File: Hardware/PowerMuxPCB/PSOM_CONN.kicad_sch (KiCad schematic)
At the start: 31 parts, among them J1 SLIMSTACK, Q2 SQ2315CES-T1_GE3, Q3 SQ2315CES-T1_GE3, Q4 SQ2315CES-T1_GE3, Q5 SQ2315CES-T1_GE3, Q6 SQ2315CES-T1_GE3, Q7 SQ2315CES-T1_GE3

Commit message: silk + roosters
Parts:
- Q2, Q3, Q4, Q5, Q6, Q7: footprint footprints1:PMOSGSD_SOT-23_TO-236_VIS -> PMOSGSD_SOT-23_TO-236_VIS
- TP11: footprint TestPoint:TestPoint_Pad_D2.0mm -> TestPoint:TestPoint_THTPad_D2.0mm_Drill1.0mm
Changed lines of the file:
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@@
 			)
 		)
-		(property "Footprint" "TestPoint:TestPoint_Pad_D2.0mm"
+		(property "Footprint" "TestPoint:TestPoint_THTPad_D2.0mm_Drill1.0mm"
 			(at 144.78 77.47 0)
 			(effects
@@
 			)
 		)
-		(property "Footprint" "footprints1:PMOSGSD_SOT-23_TO-236_VIS"
+		(property "Footprint" "PMOSGSD_SOT-23_TO-236_VIS"
 			(at 208.28 49.53 0)
 			(effects
@@
 			)
 		)
-		(property "Footprint" "footprints1:PMOSGSD_SOT-23_TO-236_VIS"
+		(property "Footprint" "PMOSGSD_SOT-23_TO-236_VIS"
 			(at 208.28 24.13 0)
 			(effects
@@
 			)
 		)
-		(property "Footprint" "footprints1:PMOSGSD_SOT-23_TO-236_VIS"
+		(property "Footprint" "PMOSGSD_SOT-23_TO-236_VIS"
 			(at 184.15 24.13 0)
 			(effects
@@
 			)
 		)
-		(property "Footprint" "footprints1:PMOSGSD_SOT-23_TO-236_VIS"
+		(property "Footprint" "PMOSGSD_SOT-23_TO-236_VIS"
 			(at 184.15 49.53 0)
 			(effects
@@
 			)
 		)
-		(property "Footprint" "footprints1:PMOSGSD_SOT-23_TO-236_VIS"
+		(property "Footprint" "PMOSGSD_SOT-23_TO-236_VIS"
 			(at 208.28 36.83 0)
 			(effects
@@
 			)
 		)
-		(property "Footprint" "footprints1:PMOSGSD_SOT-23_TO-236_VIS"
+		(property "Footprint" "PMOSGSD_SOT-23_TO-236_VIS"
 			(at 184.15 36.83 0)
 			(effects

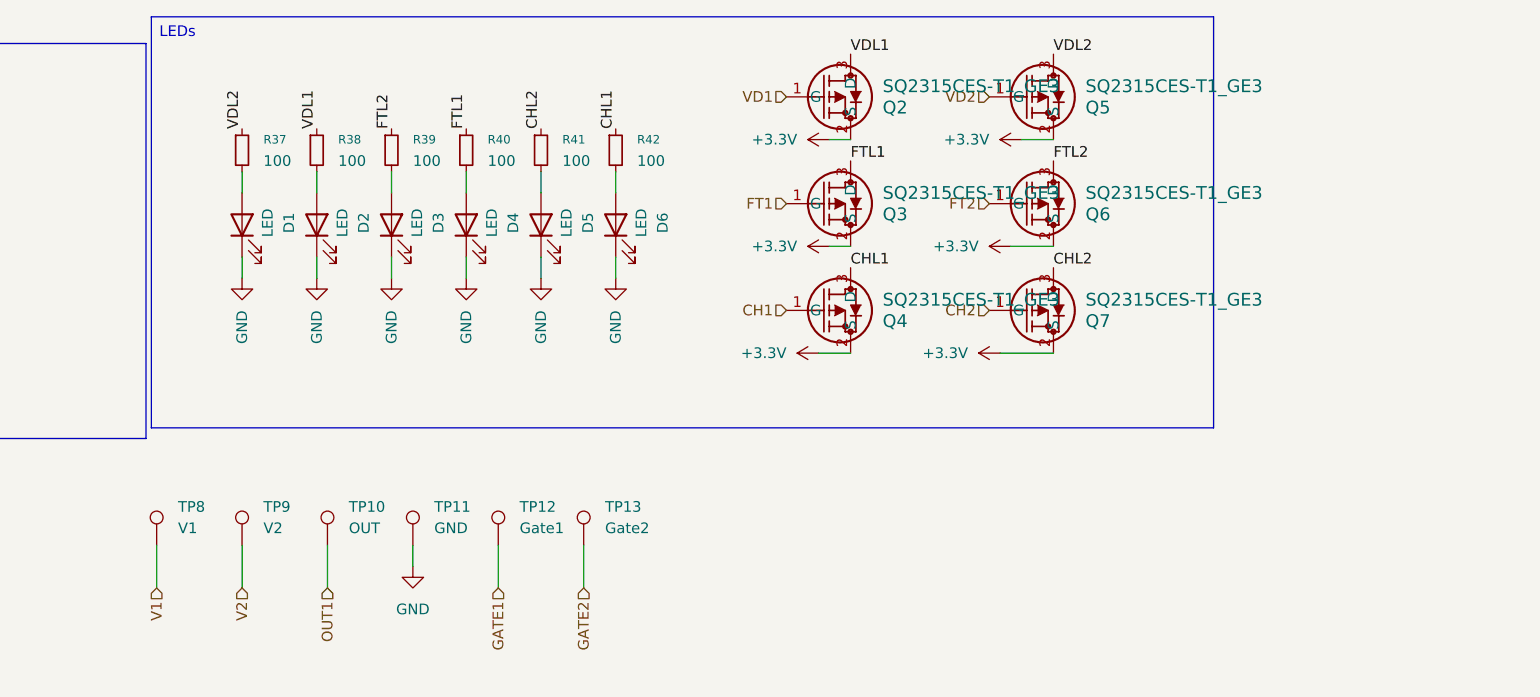
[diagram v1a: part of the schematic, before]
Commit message: cleaned up power mux
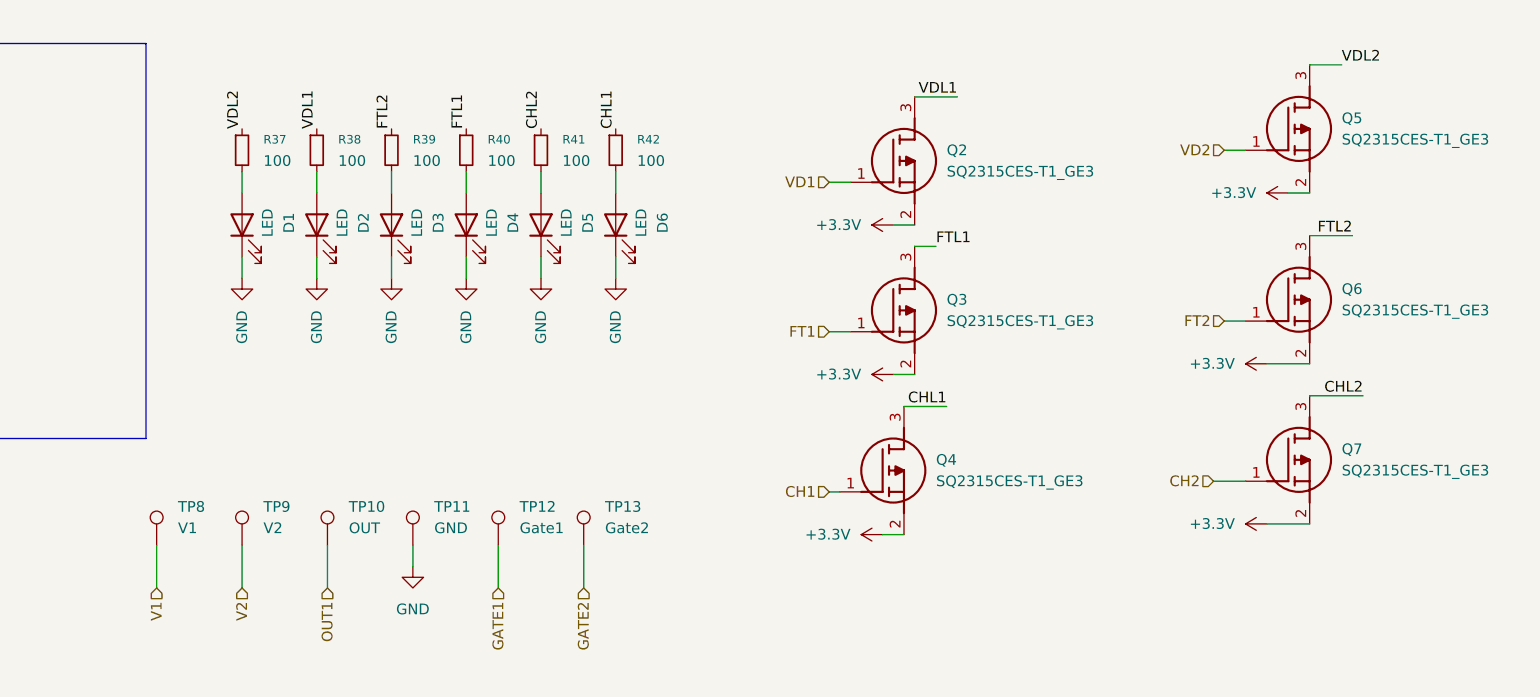
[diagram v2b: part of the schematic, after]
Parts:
- removed Q2, Q3, Q4, Q5, Q6, Q7: SQ2315CES-T1_GE3, PMOSGSD_SOT-23_TO-236_VIS, symbol sumStuff1:SQ2315CES-T1_GE3
- added Q2, Q3, Q4, Q5, Q6, Q7: SQ2315CES-T1_GE3, PowerMuxLib:SQ2315CES-T1_GE3, symbol PowerMuxLib:SQ2315CES-T1_GE3
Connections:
- net +3.3V: now also Q2.2 (S), Q3.2 (S), Q4.2 (S), Q5.2 (S), Q6.2 (S), Q7.2 (S)
- net CH1: now also Q4.1 (G)
- net CH2: now also Q7.1 (G)
- net CHL1: now also Q4.3 (D)
- net CHL2: now also Q7.3 (D)
- net FT1: now also Q3.1 (G)
- net FT2: now also Q6.1 (G)
- net FTL1: now also Q3.3 (D)
- net FTL2: now also Q6.3 (D)
- net VD1: now also Q2.1 (G)
- net VD2: now also Q5.1 (G)
- net VDL1: now also Q2.3 (D)
- net VDL2: now also Q5.3 (D)

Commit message: stared adding jlcpcb p/ns
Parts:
- J1: Manufacturer_Name Molex -> (none); Mouser Part Number 538-52465-2470 -> (none); Mouser Price/Stock https://www.mouser.co.uk/ProductDetail/Molex/52465-2470?qs=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 -> (none)
- Q2, Q3, Q4, Q5, Q6, Q7: Manufacturer_Name Vishay -> (none); Manufacturer_Part_Number SQ2315CES-T1_GE3 -> (none)
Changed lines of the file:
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@@
 			)
 		)
-		(property "Manufacturer_Name" "Vishay"
-			(at 250.19 729.21 0)
-			(effects
-				(font
-					(size 1.27 1.27)
-				)
-				(justify left top)
-				(hide yes)
-			)
-		)
-		(property "Manufacturer_Part_Number" "SQ2315CES-T1_GE3"
-			(at 250.19 829.21 0)
-			(effects
-				(font
-					(size 1.27 1.27)
-				)
-				(justify left top)
-				(hide yes)
-			)
-		)
 		(pin "1"
 		)
@@
 			)
 		)
-		(property "Manufacturer_Name" "Vishay"
-			(at 203.2 750.8 0)
-			(effects
-				(font
-					(size 1.27 1.27)
-				)
-				(justify left top)
-				(hide yes)
-			)
-		)
-		(property "Manufacturer_Part_Number" "SQ2315CES-T1_GE3"
-			(at 203.2 850.8 0)
-			(effects
-				(font
-					(size 1.27 1.27)
-				)
-				(justify left top)
-				(hide yes)
-			)
-		)
 		(pin "1"
 		)
@@
 			)
 		)
-		(property "Manufacturer_Name" "Vishay"
-			(at 250.19 749.53 0)
-			(effects
-				(font
-					(size 1.27 1.27)
-				)
-				(justify left top)
-				(hide yes)
-			)
-		)
-		(property "Manufacturer_Part_Number" "SQ2315CES-T1_GE3"
-			(at 250.19 849.53 0)
-			(effects
-				(font
-					(size 1.27 1.27)
-				)
-				(justify left top)
-				(hide yes)
-			)
-		)
 		(pin "1"
 		)
@@
 			)
 		)
-		(property "Manufacturer_Name" "Vishay"
-			(at 203.2 733.02 0)
-			(effects
-				(font
-					(size 1.27 1.27)
-				)
-				(justify left top)
-				(hide yes)
-			)
-		)
-		(property "Manufacturer_Part_Number" "SQ2315CES-T1_GE3"
-			(at 203.2 833.02 0)
-			(effects
-				(font
-					(size 1.27 1.27)
-				)
-				(justify left top)
-				(hide yes)
-			)
-		)
 		(pin "1"
 		)
@@
 			)
 		)
-		(property "Mouser Part Number" "538-52465-2470"
-			(at 53.34 522.86 0)
-			(effects
-				(font
-					(size 1.27 1.27)
-				)
-				(justify left top)
-				(hide yes)
-			)
-		)
-		(property "Mouser Price/Stock" "https://www.mouser.co.uk/ProductDetail/Molex/52465-2470?qs=sEN%2FkO1EG6Yhu4DkZwbE7Q%3D%3D"
-			(at 53.34 622.86 0)
-			(effects
-				(font
-					(size 1.27 1.27)
-				)
-				(justify left top)
-				(hide yes)
-			)
-		)
-		(property "Manufacturer_Name" "Molex"
-			(at 53.34 722.86 0)
-			(effects
-				(font
-					(size 1.27 1.27)
-				)
-				(justify left top)
-				(hide yes)
-			)
-		)
 		(property "P/N" "52465-2470"
 			(at 53.34 822.86 0)
@@
 			)
 		)
-		(property "Manufacturer_Name" "Vishay"
-			(at 201.93 769.85 0)
-			(effects
-				(font
-					(size 1.27 1.27)
-				)
-				(justify left top)
-				(hide yes)
-			)
-		)
-		(property "Manufacturer_Part_Number" "SQ2315CES-T1_GE3"
-			(at 201.93 869.85 0)
-			(effects
-				(font
-					(size 1.27 1.27)
-				)
-				(justify left top)
-				(hide yes)
-			)
-		)
 		(pin "1"
 		)
@@
 			(effects
 				(font
-					(size 1.27 1.27)
-				)
-				(justify left top)
-				(hide yes)
-			)
-		)
-		(property "Manufacturer_Name" "Vishay"
-			(at 250.19 768.58 0)
-			(effects
-				(font
-					(size 1.27 1.27)
-				)
-				(justify left top)
-				(hide yes)
-			)
-		)
-		(property "Manufacturer_Part_Number" "SQ2315CES-T1_GE3"
-			(at 250.19 868.58 0)
-			(effects
-				(font

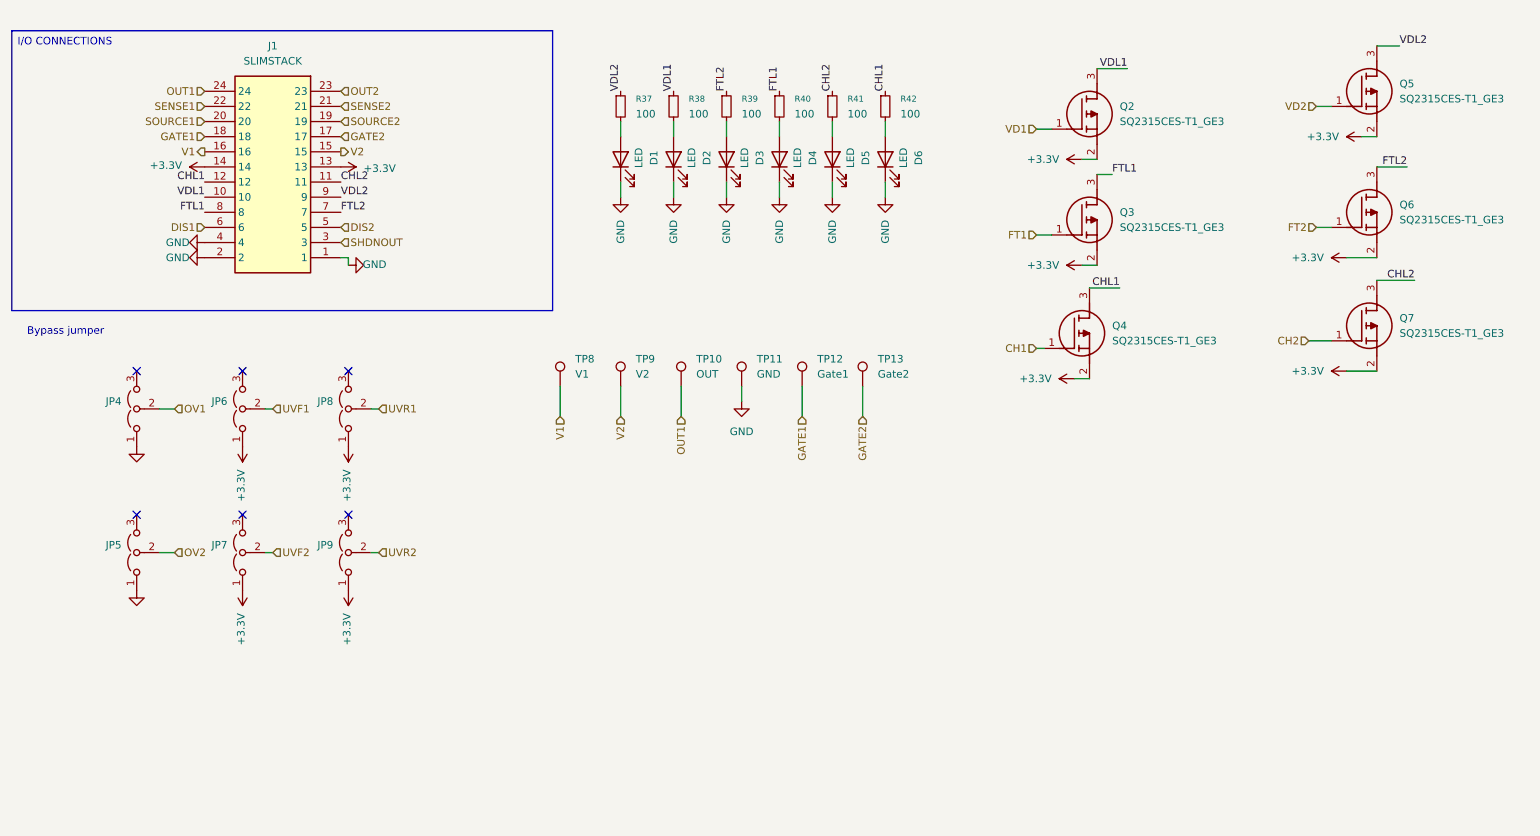
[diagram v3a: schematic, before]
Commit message: mostly done w/ rev b
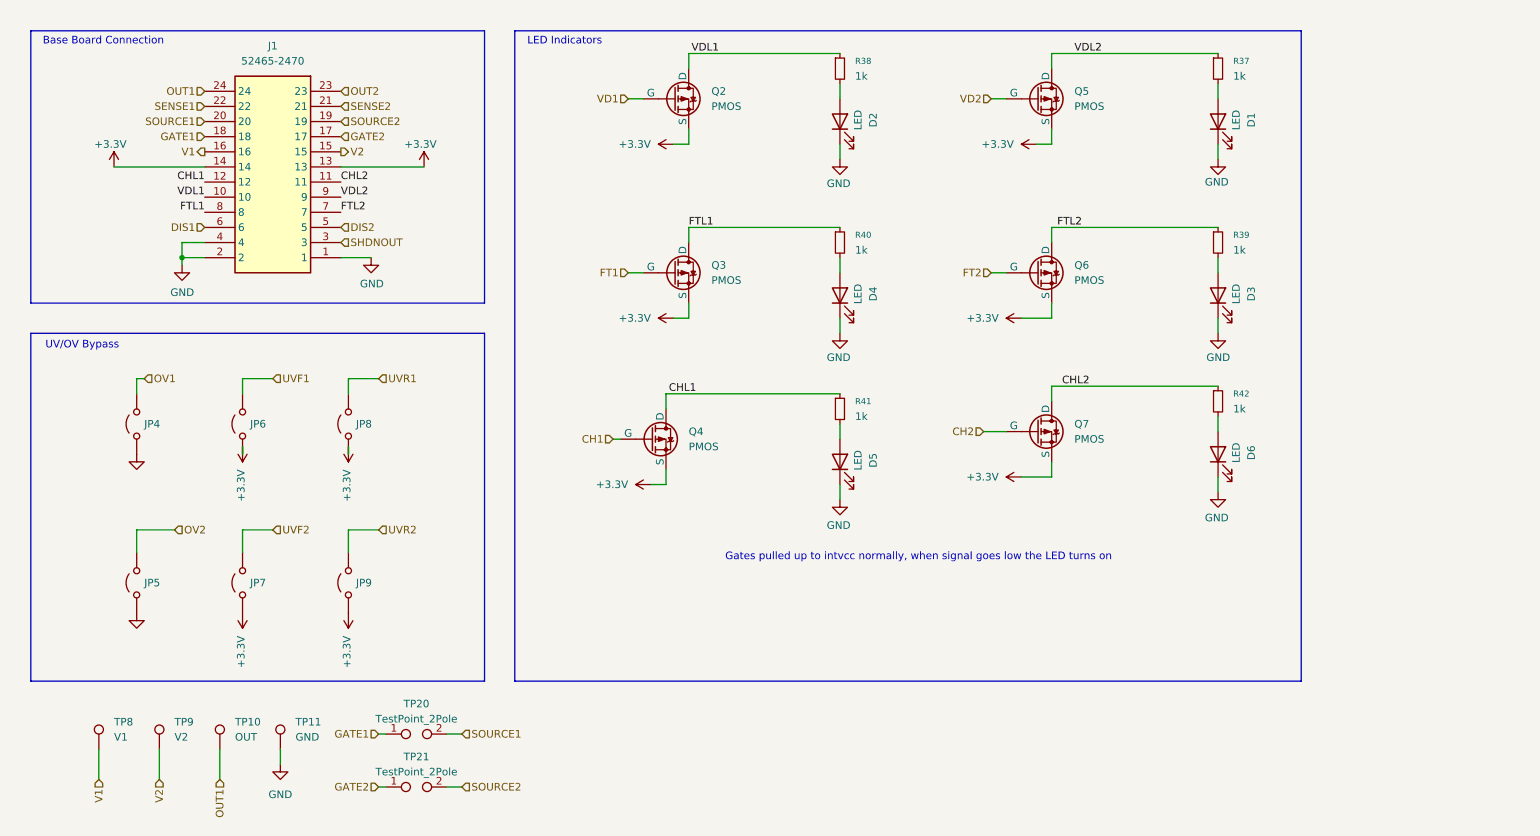
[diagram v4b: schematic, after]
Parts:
- removed JP4, JP5, JP6, JP7, JP8, JP9: ~, Connector_PinHeader_2.54mm:PinHeader_1x03_P2.54mm_Vertical, symbol Jumper:Jumper_3_Open
- removed Q2, Q3, Q4, Q5, Q6, Q7: SQ2315CES-T1_GE3, PowerMuxLib:SQ2315CES-T1_GE3, symbol PowerMuxLib:SQ2315CES-T1_GE3
- removed TP12: Gate1, TestPoint:TestPoint_Pad_D2.0mm, symbol Connector:TestPoint
- removed TP13: Gate2, TestPoint:TestPoint_Pad_D2.0mm, symbol Connector:TestPoint
- added JP4, JP5, JP6, JP7, JP8, JP9: Jumper_2_Open, Connector_PinHeader_2.54mm:PinHeader_1x02_P2.54mm_Vertical, symbol Jumper:Jumper_2_Open
- added Q2, Q3, Q4, Q5, Q6, Q7: PMOS, PowerMuxLib:IRLML5203TRPBF, symbol Simulation_SPICE:PMOS
- added TP20, TP21: TestPoint_2Pole, TestPoint:TestPoint_2Pads_Pitch2.54mm_Drill0.8mm, symbol Connector:TestPoint_2Pole
- J1: value SLIMSTACK -> 52465-2470
- R37, R38, R39, R40, R41, R42: value 100 -> 1k
- TP10, TP8, TP9: footprint TestPoint:TestPoint_Pad_D2.0mm -> TestPoint:TestPoint_Plated_Hole_D2.0mm; now left out of the parts list
- TP11: footprint TestPoint:TestPoint_THTPad_D2.0mm_Drill1.0mm -> TestPoint:TestPoint_Plated_Hole_D2.0mm; now left out of the parts list
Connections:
- net +3.3V: now also JP6.1 (A), JP7.1 (A), JP8.1 (A), JP9.1 (A), Q2.3 (S), Q3.3 (S), Q4.3 (S), Q5.3 (S), Q6.3 (S), Q7.3 (S)
- net CH1: now also Q4.2 (G)
- net CH2: now also Q7.2 (G)
- net CHL1: now also R41.1, Q4.1 (D); no longer R42.1
- net CHL2: now also R42.1, Q7.1 (D); no longer R41.1
- net FT1: now also Q3.2 (G)
- net FT2: now also Q6.2 (G)
- net FTL1: now also Q3.1 (D)
- net FTL2: now also Q6.1 (D)
- net GATE1: now also TP20.1
- net GATE2: now also TP21.1
- net GND: now also JP4.1 (A), JP5.1 (A)
- net OV1: now also JP4.2 (B)
- net OV2: now also JP5.2 (B)
- net SOURCE1: now also TP20.2
- net SOURCE2: now also TP21.2
- net UVF1: now also JP6.2 (B)
- net UVF2: now also JP7.2 (B)
- net UVR1: now also JP8.2 (B)
- net UVR2: now also JP9.2 (B)
- net VD1: now also Q2.2 (G)
- net VD2: now also Q5.2 (G)
- net VDL1: now also Q2.1 (D)
- net VDL2: now also Q5.1 (D)
- no-connect marks 6 -> 0
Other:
- note added: "Base Board Connection"
- note added: "Gates pulled up to intvcc normally, when signal goes low the LED turns on"
- note added: "LED Indicators"
- note added: "UV/OV Bypass"
- note removed: "Bypass jumper"
- moved on the sheet: D1, D2, D3, D4, D5, D6, R37, R38, R39, R40, R41, R42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
